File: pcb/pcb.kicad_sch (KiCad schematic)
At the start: 49 parts, among them CN1 Battery_Cell, Q1 2N7002, Q2 AO3401A, Q3 AO3400A, U1 USB-C 6PIN, U2 TPS63802DLAT, U3 BQ24075RGTR, U4 TUSB320LIRWBR, U5 ESP-32S DevBoard, U6 Water_Sensor, U7 Pump

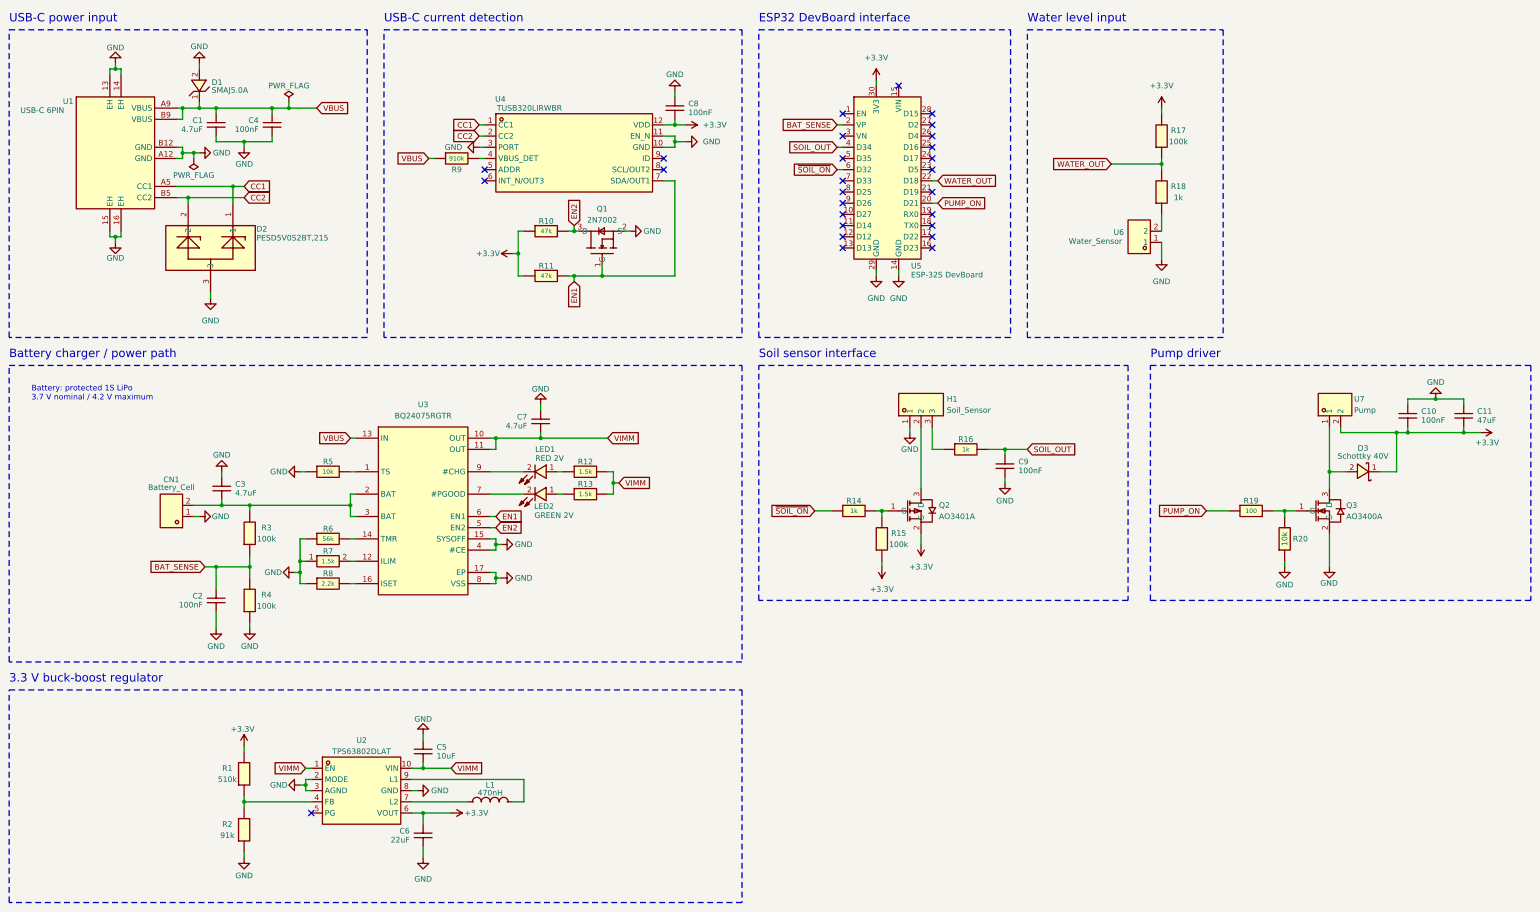
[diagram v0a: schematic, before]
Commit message: Fixed the PCB design
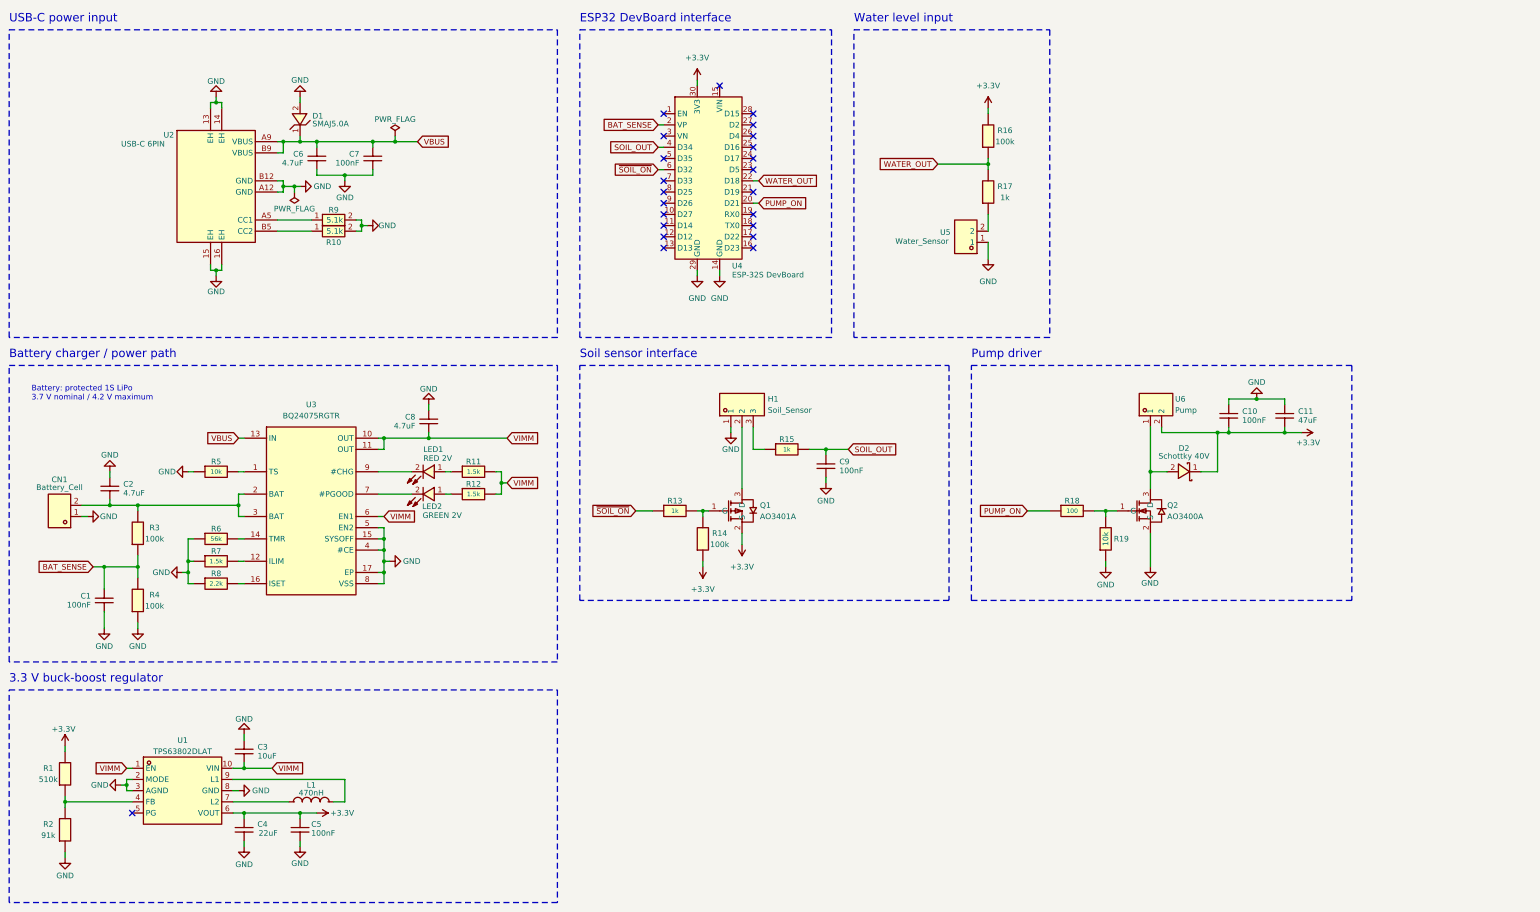
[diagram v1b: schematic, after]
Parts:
- removed C8: 100nF, EasyEDA:C0805, symbol EasyEDA:0805C 100nF
- removed D2: PESD5V0S2BT,215, EasyEDA:SOT-23_L2.9-W1.3-P1.90-LS2.4-BR, symbol EasyEDA:PESD5V0S2BT,215
- removed Q1: 2N7002, EasyEDA:SOT-23-3_L2.9-W1.3-P1.90-LS2.4-BR, symbol EasyEDA:SOT-23 2N7002
- removed R10, R11: 47k, EasyEDA:R0805, symbol EasyEDA:0805R 47k
- removed R9: 910k, EasyEDA:R0805, symbol EasyEDA:0805R 900k
- removed U4: TUSB320LIRWBR, EasyEDA:X2QFN-12_L1.6-W1.6-P0.40-TL, symbol EasyEDA:TUSB320IRWBR
- added C5: 100nF, EasyEDA:C0805, symbol EasyEDA:0805C 100nF
- added R10, R9: 5.1k, EasyEDA:R0805, symbol EasyEDA:0805R 5.1k
- C11: LCSC Part C16780 -> C141660; MPN CL21A476MQYNNNE -> GRM21BR60J107ME15L; Manufacturer SAMSUNG(三星) -> muRata(村田)
- C4: renamed from C6; LCSC Part C45783 -> C29277; MPN CL21A226MAQNNNE -> CL21A226MPQNNNE
- D1: LCSC Part C2925443 -> C223993; MPN SMAJ5.0A -> SMAJ6.0A; Manufacturer Liown -> Littelfuse(美国力特)
- R7: LCSC Part C4310 -> C2933331; MPN 0805W8F1501T5E -> FRC0805F1621TS; Manufacturer UNI-ROYAL(厚声) -> FOJAN(富捷)
- renumbered C2 to C1, C3 to C2, C5 to C3, C1 to C6, C4 to C7, C7 to C8, D3 to D2, Q2 to Q1, Q3 to Q2, R12 to R11, R13 to R12, R14 to R13, R15 to R14, R16 to R15, R17 to R16, R18 to R17, R19 to R18, R20 to R19, U2 to U1, U1 to U2, U5 to U4, U6 to U5, U7 to U6
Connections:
- net EN1 is gone; now on net VIMM: U3.6 (EN1)
- net EN2 is gone; now on net GND: U3.5 (EN2)
- net +3.3V: now also C5.1
- net GND: now also C5.2, R10.2, R9.2
- net CC1: no longer names the net of U2.A5 (CC1)
- net CC1: now also R9.1
- net CC2: no longer names the net of U2.B5 (CC2)
- net CC2: now also R10.1
- no-connect marks 27 -> 23
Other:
- note removed: "USB-C current detection"
- moved on the sheet: C1, C10, C11, C2, C3, C4, C6, C7, C8, C9, CN1, D1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
